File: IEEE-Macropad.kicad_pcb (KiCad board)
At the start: 2 copper layers, 98.4 x 76.2 mm, 48 parts, among them SW1 SW_Push, U1 ATmega32U4-A, Y1 16MHz

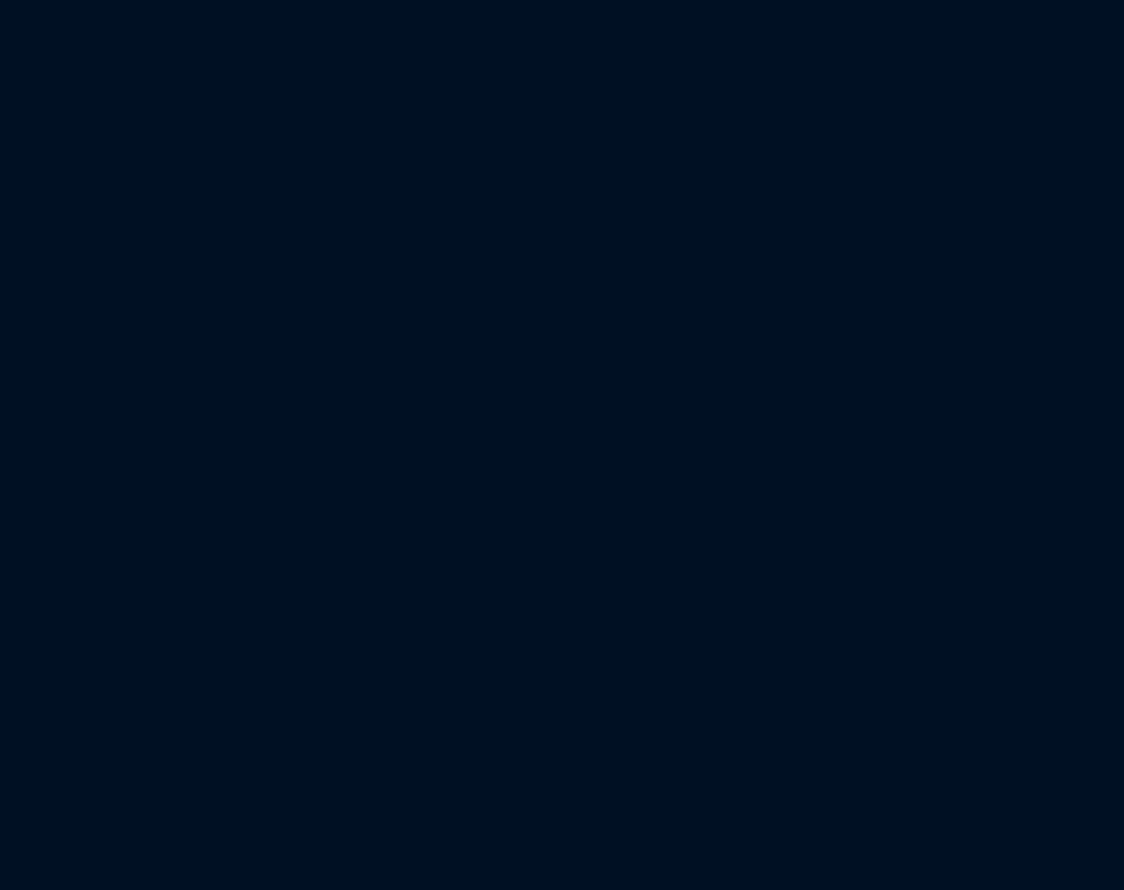
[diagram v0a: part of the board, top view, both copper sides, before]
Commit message: Add files via upload
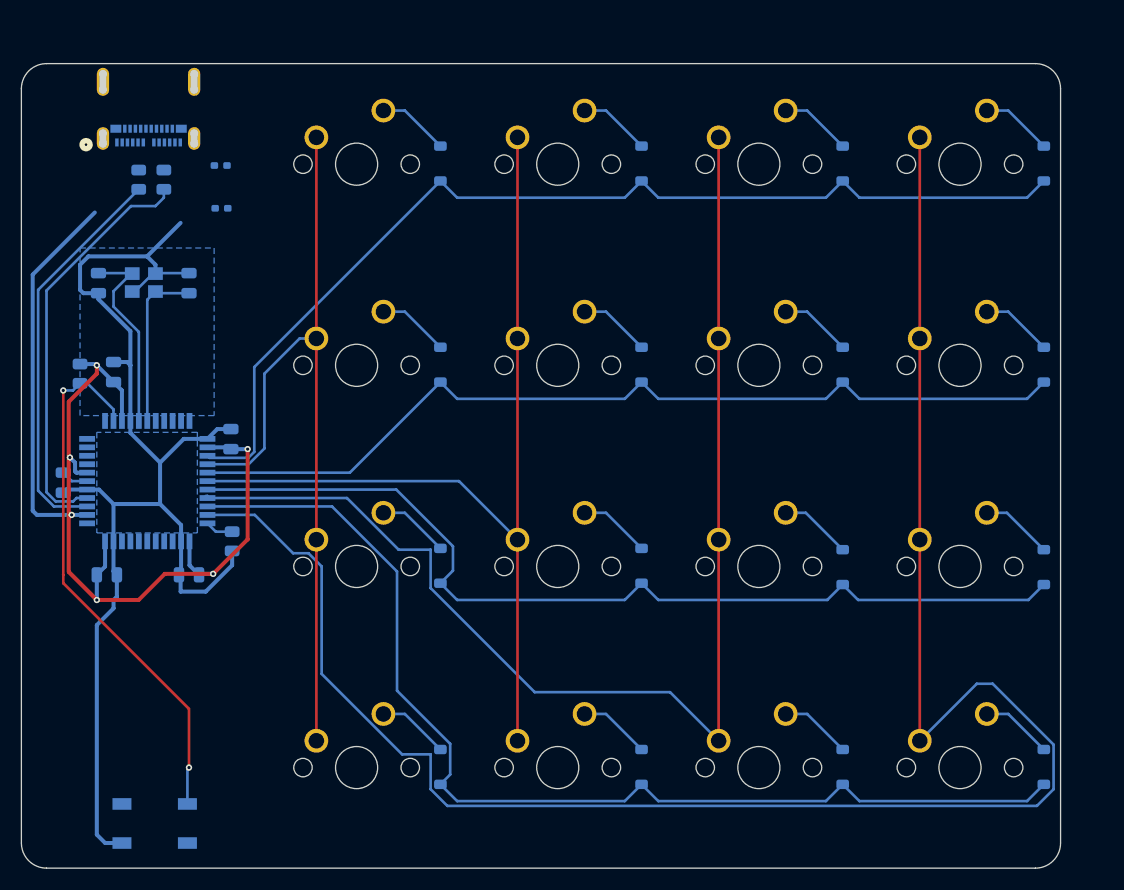
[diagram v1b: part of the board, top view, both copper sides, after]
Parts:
- added C1: 22pF, Capacitor_SMD:C_0805_2012Metric, B.Cu at (64.0, 130.3)
- added C2: 22pF, Capacitor_SMD:C_0805_2012Metric, B.Cu at (55.4, 130.3)
- added C3: 1uF, Capacitor_SMD:C_0805_2012Metric, B.Cu at (52.1, 149.2)
- added C4: 0.1uF, Capacitor_SMD:C_0805_2012Metric, B.Cu at (67.9, 145.1)
- added C5: 0.1uF, Capacitor_SMD:C_0805_2012Metric, B.Cu at (56.8, 138.7)
- added C6: 0.1uF, Capacitor_SMD:C_0805_2012Metric, B.Cu at (64.0, 157.9)
- added C7: 10uF, Capacitor_SMD:C_0805_2012Metric, B.Cu at (56.2, 157.9)
- added D1: SOD-123, Diode_SMD:D_SOD-123, B.Cu at (87.8, 119.0)
- added D10: SOD-123, Diode_SMD:D_SOD-123, B.Cu at (106.8, 157.1)
- added D11: SOD-123, Diode_SMD:D_SOD-123, B.Cu at (125.9, 157.2)
- added D12: SOD-123, Diode_SMD:D_SOD-123, B.Cu at (144.9, 157.2)
- added D13: SOD-123, Diode_SMD:D_SOD-123, B.Cu at (87.8, 176.1)
- added D14: SOD-123, Diode_SMD:D_SOD-123, B.Cu at (106.8, 176.1)
- added D15: SOD-123, Diode_SMD:D_SOD-123, B.Cu at (125.9, 176.1)
- added D16: SOD-123, Diode_SMD:D_SOD-123, B.Cu at (144.9, 176.1)
- added D2: SOD-123, Diode_SMD:D_SOD-123, B.Cu at (106.8, 119.0)
- added D3: SOD-123, Diode_SMD:D_SOD-123, B.Cu at (125.9, 119.0)
- added D4: SOD-123, Diode_SMD:D_SOD-123, B.Cu at (144.9, 119.0)
- added D5: SOD-123, Diode_SMD:D_SOD-123, B.Cu at (87.8, 138.0)
- added D6: SOD-123, Diode_SMD:D_SOD-123, B.Cu at (106.8, 138.0)
- added D7: SOD-123, Diode_SMD:D_SOD-123, B.Cu at (125.9, 138.0)
- added D8: SOD-123, Diode_SMD:D_SOD-123, B.Cu at (144.9, 138.0)
- added D9: SOD-123, Diode_SMD:D_SOD-123, B.Cu at (87.8, 157.1)
- added MX1: MX-NoLED, MX_Only:MXOnly-1U-NoLED, F.Cu at (79.8, 119.0)
- added MX10: MX-NoLED, MX_Only:MXOnly-1U-NoLED, F.Cu at (98.9, 157.1)
- added MX11: MX-NoLED, MX_Only:MXOnly-1U-NoLED, F.Cu at (117.9, 157.1)
- added MX12: MX-NoLED, MX_Only:MXOnly-1U-NoLED, F.Cu at (137.0, 157.1)
- added MX13: MX-NoLED, MX_Only:MXOnly-1U-NoLED, F.Cu at (79.8, 176.2)
- added MX14: MX-NoLED, MX_Only:MXOnly-1U-NoLED, F.Cu at (98.9, 176.2)
- added MX15: MX-NoLED, MX_Only:MXOnly-1U-NoLED, F.Cu at (117.9, 176.2)
- added MX16: MX-NoLED, MX_Only:MXOnly-1U-NoLED, F.Cu at (137.0, 176.2)
- added MX2: MX-NoLED, MX_Only:MXOnly-1U-NoLED, F.Cu at (98.9, 119.0)
- added MX3: MX-NoLED, MX_Only:MXOnly-1U-NoLED, F.Cu at (117.9, 119.0)
- added MX4: MX-NoLED, MX_Only:MXOnly-1U-NoLED, F.Cu at (137.0, 119.0)
- added MX5: MX-NoLED, MX_Only:MXOnly-1U-NoLED, F.Cu at (79.8, 138.1)
- added MX6: MX-NoLED, MX_Only:MXOnly-1U-NoLED, F.Cu at (98.9, 138.1)
- added MX7: MX-NoLED, MX_Only:MXOnly-1U-NoLED, F.Cu at (117.9, 138.1)
- added MX8: MX-NoLED, MX_Only:MXOnly-1U-NoLED, F.Cu at (137.0, 138.1)
- added MX9: MX-NoLED, MX_Only:MXOnly-1U-NoLED, F.Cu at (79.8, 157.1)
- added R1: 10k, Resistor_SMD:R_0805_2012Metric, B.Cu at (53.7, 138.9)
- added R2: 22, Resistor_SMD:R_0805_2012Metric, B.Cu at (61.6, 120.5)
- added R3: 22, Resistor_SMD:R_0805_2012Metric, B.Cu at (59.2, 120.5)
- added R4: 10k, Resistor_SMD:R_0805_2012Metric, B.Cu at (68.1, 154.8)
- added R5: 5.1k, Resistor_SMD:R_0402_1005Metric_Pad0.72x0.64mm_HandSolder, B.Cu at (67.0, 119.2)
- added R6: 5.1k, Resistor_SMD:R_0402_1005Metric_Pad0.72x0.64mm_HandSolder, B.Cu at (67.0, 123.2)
- added SW1: SW_Push, random-keyboard-parts:SKQG-1155865, B.Cu at (60.7, 181.5)
- added U1: ATmega32U4-A, Package_QFP:TQFP-44_10x10mm_P0.8mm, B.Cu at (60.0, 149.1)
- added USB2: Molex-1054500101, footprints:CONN_105450-0101_MOL, B.Cu at (60.1, 113.2)
- added Y1: 16MHz, Crystal:Crystal_SMD_3225-4Pin_3.2x2.5mm, B.Cu at (59.7, 130.3)
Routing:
- net COL3: track 178.8 -> 357.5 mm
- net COL2: track 117.6 -> 235.2 mm
- net GND: track 126.6 -> 244.1 mm
- net +5V: track 111.2 -> 222.5 mm, vias 6 -> 12
- net ROW3: track 104.2 -> 208.5 mm
- net ROW0: track 98.8 -> 197.6 mm
- net ROW2: track 90.4 -> 180.8 mm
- net COL1: track 88.8 -> 177.6 mm
- net ROW1: track 86.7 -> 173.4 mm
- net COL0: track 76.5 -> 153.1 mm
- net Net-(U1-~{RESET}): track 51.3 -> 102.6 mm, vias 2 -> 4
- net Net-(U1-D+): track 39.0 -> 78.0 mm
- net Net-(U1-D-): track 37.7 -> 75.5 mm
- net Net-(U1-XTAL2): track 19.0 -> 37.9 mm
- net Net-(U1-XTAL1): track 15.8 -> 31.6 mm
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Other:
- board size 98.4 x 76.2 mm -> 175.7 x 161.1 mm
